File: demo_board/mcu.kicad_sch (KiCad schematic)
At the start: 10 parts, among them U5 BME280, U6 LSM6DS3

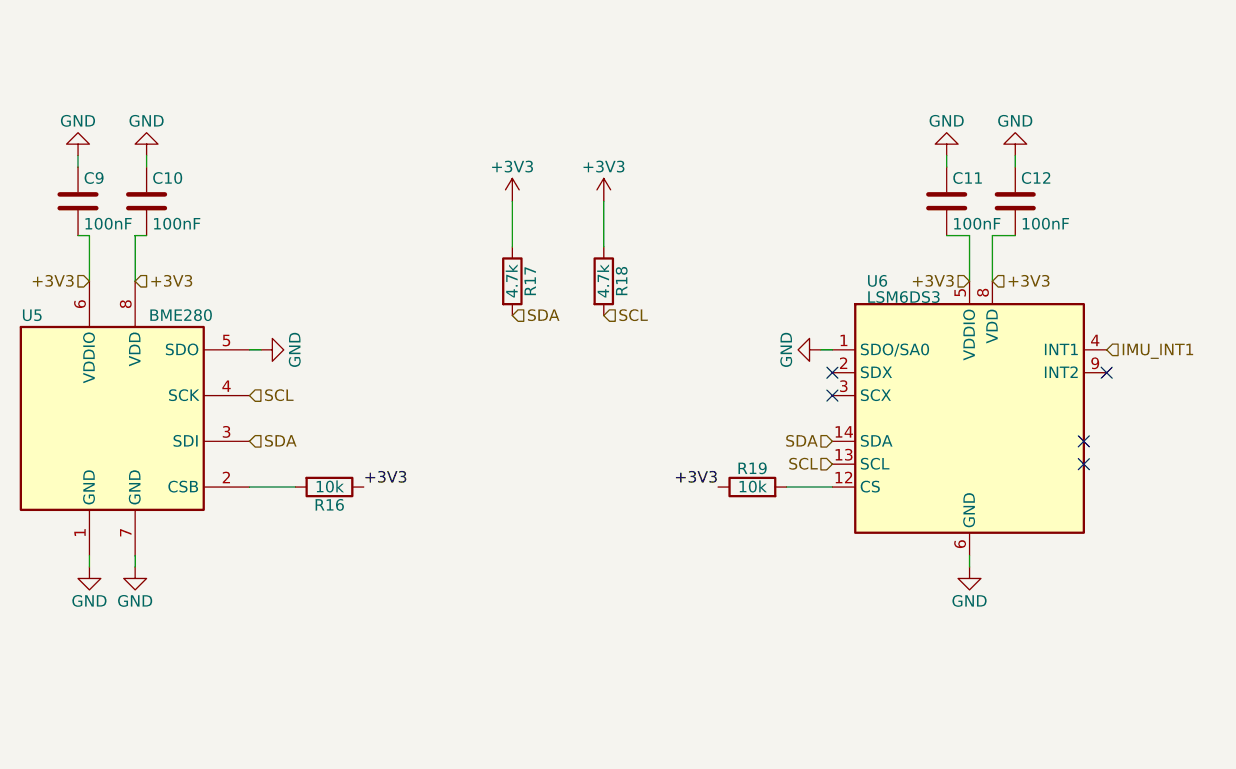
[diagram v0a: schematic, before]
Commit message: new demo board
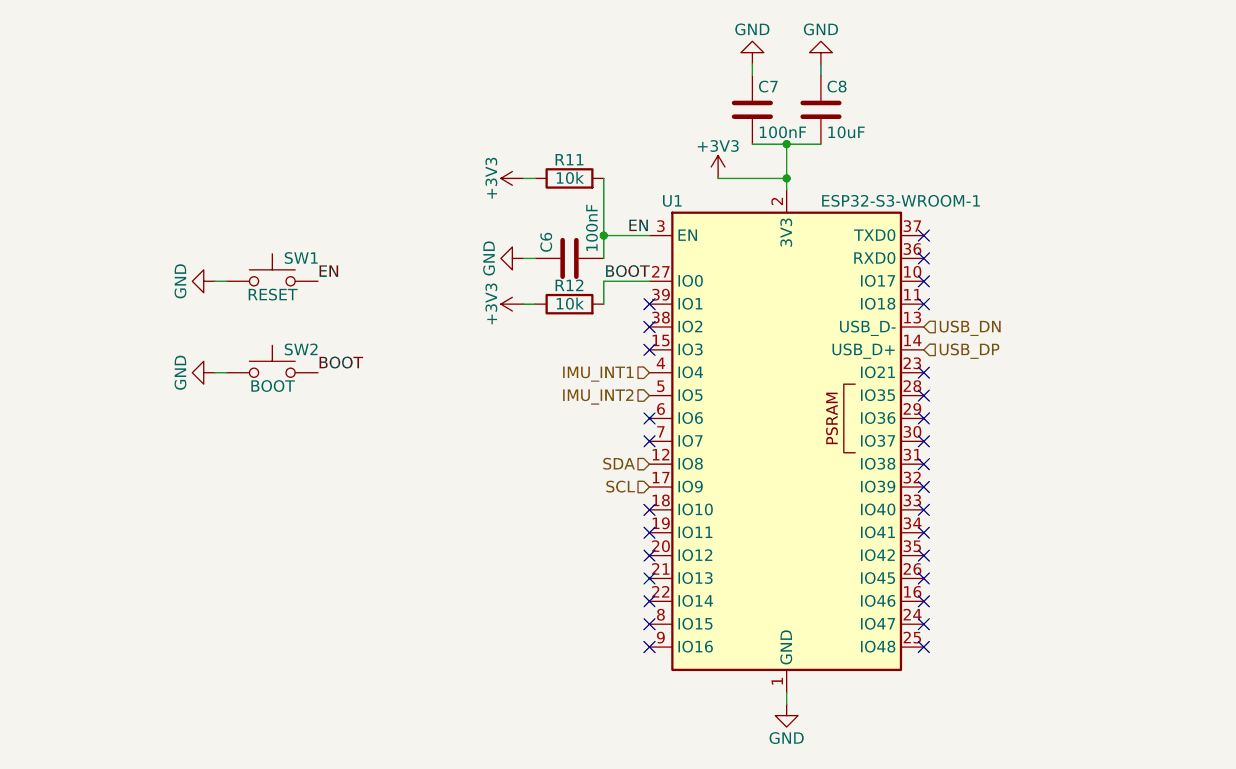
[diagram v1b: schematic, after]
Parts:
- removed C10, C11, C12, C9: 100nF, Capacitor_SMD:C_0402_1005Metric, symbol Device:C
- removed R16, R19: 10k, Resistor_SMD:R_0402_1005Metric, symbol Device:R
- removed R17, R18: 4.7k, Resistor_SMD:R_0402_1005Metric, symbol Device:R
- removed U5: BME280, Package_LGA:Bosch_LGA-8_2.5x2.5mm_P0.65mm_ClockwisePinNumbering, symbol Sensor:BME280
- removed U6: LSM6DS3, Package_LGA:LGA-14_3x2.5mm_P0.5mm_LayoutBorder3x4y, symbol Sensor_Motion:LSM6DS3
- added C6, C7: 100nF, Capacitor_SMD:C_0402_1005Metric, symbol Device:C
- added C8: 10uF, Capacitor_SMD:C_0805_2012Metric, symbol Device:C
- added R11, R12: 10k, Resistor_SMD:R_0603_1608Metric, symbol Device:R
- added SW1: RESET, Button_Switch_SMD:SW_SPST_B3U-1000P-B, symbol Switch:SW_Push
- added SW2: BOOT, Button_Switch_SMD:SW_SPST_B3U-1000P-B, symbol Switch:SW_Push
- added U1: ESP32-S3-WROOM-1, RF_Module:ESP32-S3-WROOM-1, symbol RF_Module:ESP32-S3-WROOM-1
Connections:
- net +3V3: now also C7.2, C8.2, R11.1, R12.1, U1.2 (3V3)
- net GND: now also C6.1, C7.1, C8.1, SW1.1, SW2.1, U1.1 (GND), U1.40 (GND), U1.41 (GND)
- net IMU_INT1: now also U1.4 (IO4)
- net SCL: now also U1.17 (IO9)
- net SDA: now also U1.12 (IO8)
- new net BOOT: R12.2, SW2.2, U1.27 (IO0)
- new net EN: C6.2, R11.2, SW1.2, U1.3 (EN)
- new net IMU_INT2: U1.5 (IO5)
- new net USB_DN: U1.13 (USB_D-)
- new net USB_DP: U1.14 (USB_D+)
- no-connect marks 5 -> 29
